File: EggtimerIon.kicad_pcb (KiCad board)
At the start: 4 copper layers, 40 x 25 mm, 26 parts, among them J1 Conn_01x02, J2 Conn_01x03, J3 B2B-PH-K-S, Q1 IRLML6244, U1 ESP32-WROOM-32-N4, U2 MPU-6050, U3 MS5611-01BA, U4 CAT24C512XI-T2, U5 AP2112K-3.3

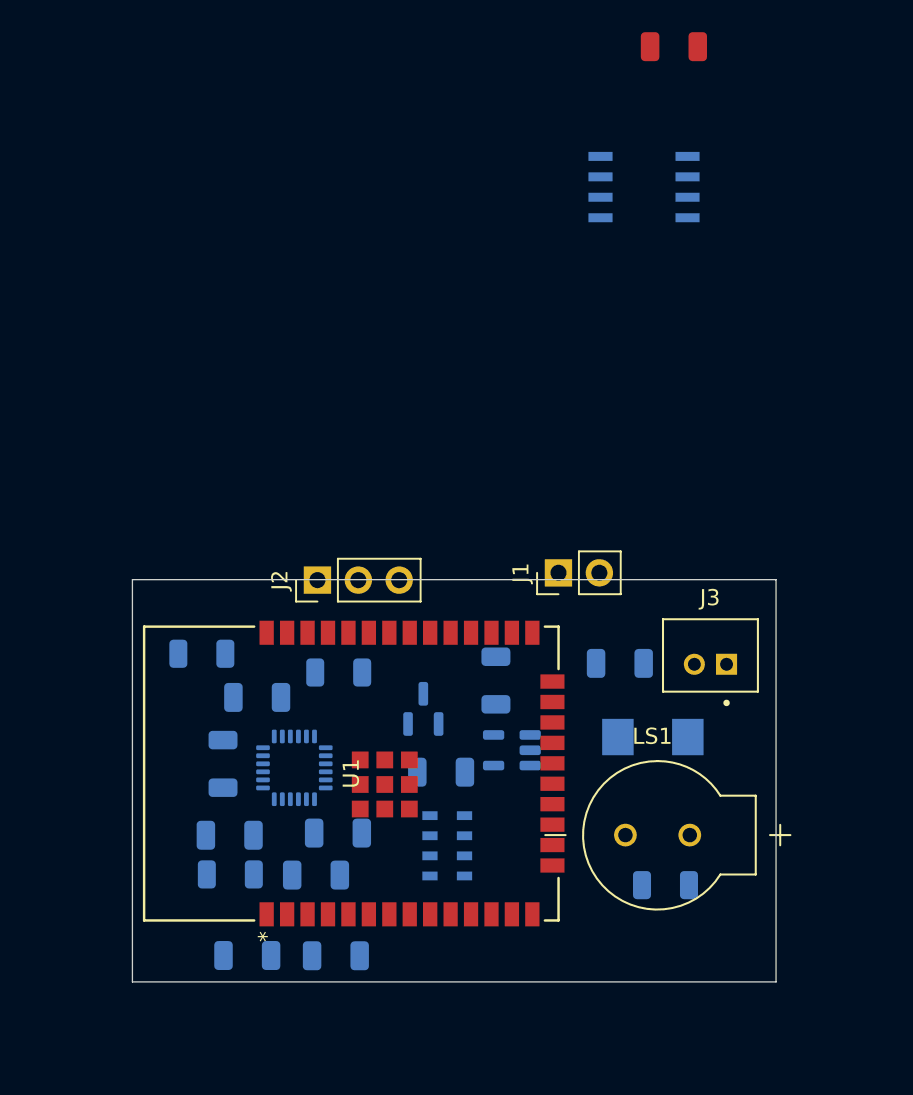
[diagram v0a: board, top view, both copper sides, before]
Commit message: Completed first round of layout
Did a lot of stuff here ok?
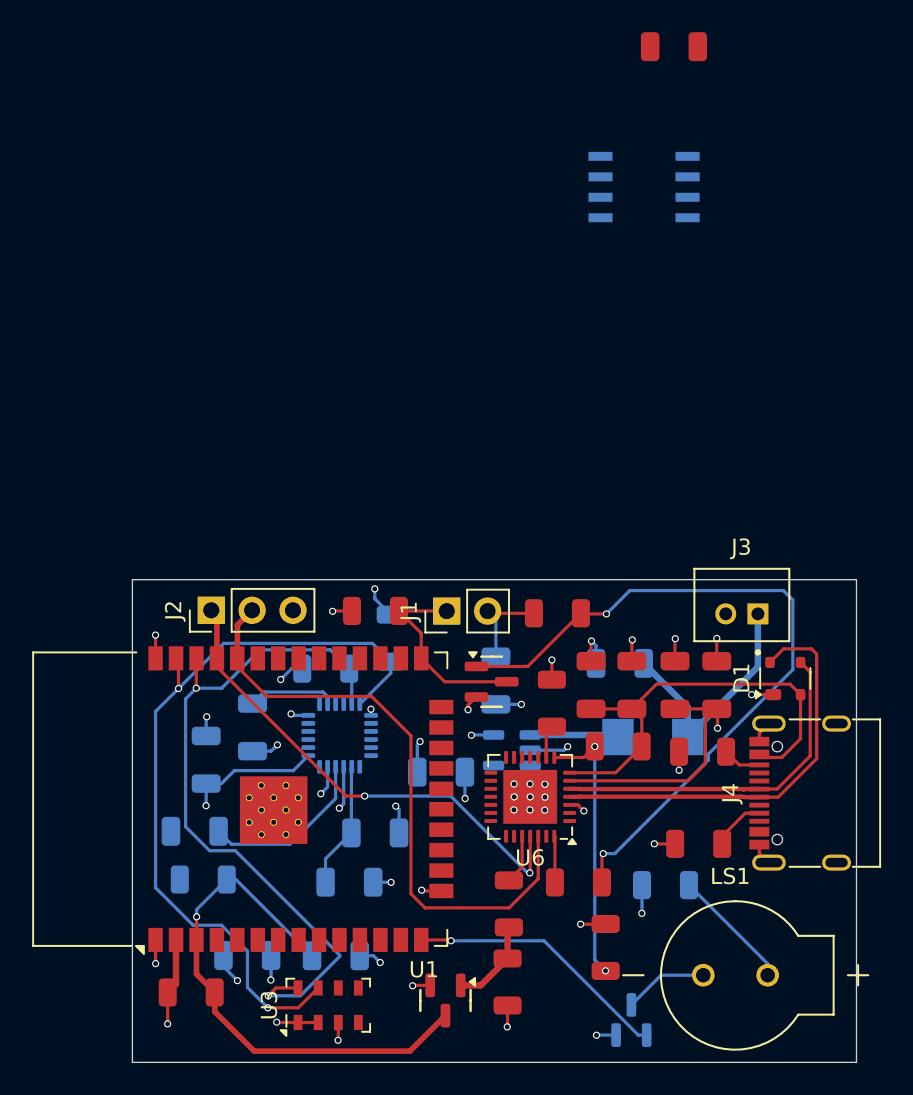
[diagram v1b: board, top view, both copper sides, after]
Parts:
- added C12: 4.7uF, PCM_JLCPCB:C_1206, F.Cu at (164.2, 91.9)
- added C13: 0.1uF, PCM_JLCPCB:C_1206, F.Cu at (166.7, 91.9)
- added C14: 4.7uF, PCM_JLCPCB:C_1206, F.Cu at (169.4, 91.9)
- added C15: 0.1uF, PCM_JLCPCB:C_1206, F.Cu at (172.0, 91.9)
- added D1: SP0503BAHT, Package_TO_SOT_SMD:SOT-143, F.Cu at (176.3, 91.5)
- added J4: USB_C_Receptacle_USB2.0, Connector_USB:USB_C_Receptacle_G-Switch_GT-USB-7010ASV, F.Cu at (178.4, 98.6)
- added Q2: 2N7002, PCM_JLCPCB:Q_SOT-23, F.Cu at (158.0, 91.7)
- added Q3: 2N7002, PCM_JLCPCB:Q_SOT-23, F.Cu at (155.2, 111.5)
- added R10: 10k, PCM_JLCPCB:R_1206, F.Cu at (150.8, 87.3)
- added R11: 10k, PCM_JLCPCB:R_1206, F.Cu at (139.4, 111.0)
- added R12: 100, PCM_JLCPCB:R_1206, F.Cu at (163.4, 104.1)
- added R13: 100k, PCM_JLCPCB:R_1206, F.Cu at (162.1, 87.4)
- added R14: 100k, PCM_JLCPCB:R_1206, F.Cu at (159.0, 110.3)
- added R15: 100, PCM_JLCPCB:R_1206, F.Cu at (159.1, 105.5)
- added R5: 1k, PCM_JLCPCB:R_1206, F.Cu at (161.8, 93.0)
- added R6: 22k1, PCM_JLCPCB:R_1206, F.Cu at (165.9, 95.7)
- added R7: 47k5, PCM_JLCPCB:R_1206, F.Cu at (165.1, 108.2)
- added R8: 5k1, PCM_JLCPCB:R_1206, F.Cu at (170.9, 101.7)
- added R9: 5k1, PCM_JLCPCB:R_1206, F.Cu at (171.1, 96.0)
- added U6: CP2102N-Axx-xQFN28, Package_DFN_QFN:QFN-28-1EP_5x5mm_P0.5mm_EP3.35x3.35mm, F.Cu at (160.4, 98.8)
- U1: footprint ESP32-WROOM-32-N4:MOD_ESP32-WROOM-32_EXP -> RF_Module:ESP32-WROOM-32
- U3: moved to F.Cu
- moved Q1 23.3 mm to (166.7, 112.7)
- moved U3 12.4 mm to (147.9, 111.8), turned to 90 degrees
- moved R2 11.8 mm to (151.8, 89.0), turned to -90 degrees
- moved LS1 9.96 mm to (173.2, 109.9)
- moved J1 7.34 mm to (155.2, 87.3)
- moved J2 6.86 mm to (140.6, 87.2)
- moved U1 4.23 mm to (145.4, 99.0)
- moved J3 3.69 mm to (173.6, 86.9)
- moved U2 3.46 mm to (148.6, 95.0)
- moved C4 2.32 mm to (150.8, 101.1)
- moved C7 2.18 mm to (139.6, 101.0)
- moved C1 2.12 mm to (149.2, 104.1)
- moved C6 1.88 mm to (143.2, 94.5), turned to -90 degrees
- moved R1 1.71 mm to (140.1, 104.0), turned to 0 degrees
- moved C5 1.08 mm to (140.3, 96.5)
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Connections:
- Q1 pad 1: /IO18 -> /IO12
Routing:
- net +3V3: track 0.00 -> 54.7 mm, vias 0 -> 13
- net GND: track 0.00 -> 51.6 mm, vias 0 -> 38
- net /SDA: track 0.00 -> 48.2 mm, vias 0 -> 2
- net Net-(Q2-G): track 0.00 -> 44.8 mm, vias 0 -> 2
- net /SCL: track 0.00 -> 44.5 mm, vias 0 -> 2
- net /RXD0: track 0.00 -> 37.9 mm
- net /EN: track 0.00 -> 33.0 mm, vias 0 -> 1
- net /TXD0: track 0.00 -> 30.7 mm, vias 0 -> 2
- net VBUS: track 0.00 -> 27.5 mm
- net /USB_D+: track 0.00 -> 26.3 mm
- net /USB_D-: track 0.00 -> 21.9 mm
- net Net-(U6-VBUS): track 0.00 -> 17.0 mm, vias 0 -> 2
- net /IO12: track 0.00 -> 16.5 mm, vias 0 -> 1
- net BAT+: track 0.00 -> 15.2 mm
- net /IO0: track 0.00 -> 12.4 mm
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- added copper zone on In2.Cu, net +3V3
- removed copper zone on In2.Cu, net GND
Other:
- board size 40 x 25 mm -> 45 x 30 mm
